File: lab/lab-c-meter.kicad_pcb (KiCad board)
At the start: 2 copper layers, 80 x 34.3 mm, 43 parts, among them J1 IN, J2 Barrel_Jack_Switch, J3 Conn_01x04, J4 USB_B_Mini, J5 PB, J6 PC, J7 PD, SW1 SW_Push, SW2 SW_Push, U1 LM324, U2 L7805, U3 ATmega8-16AU, Y1 16MHz

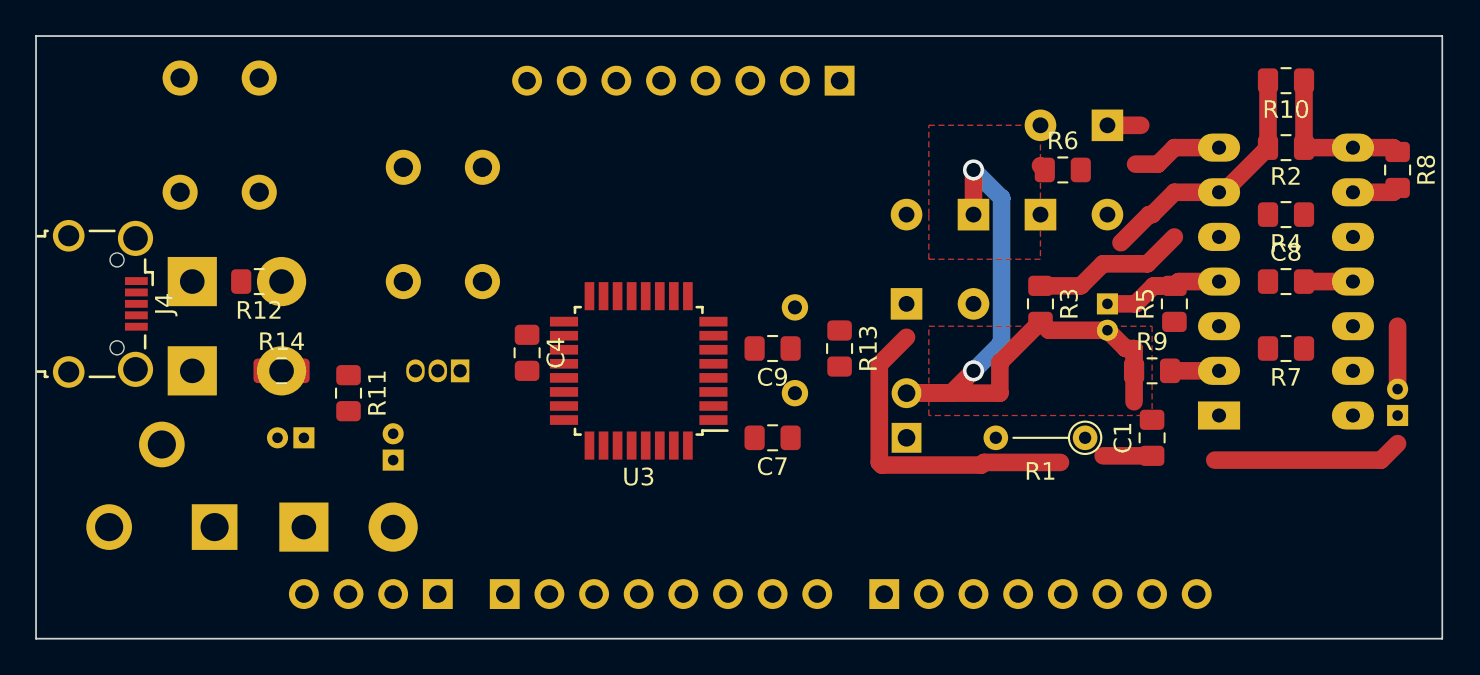
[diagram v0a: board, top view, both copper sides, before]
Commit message: Finished
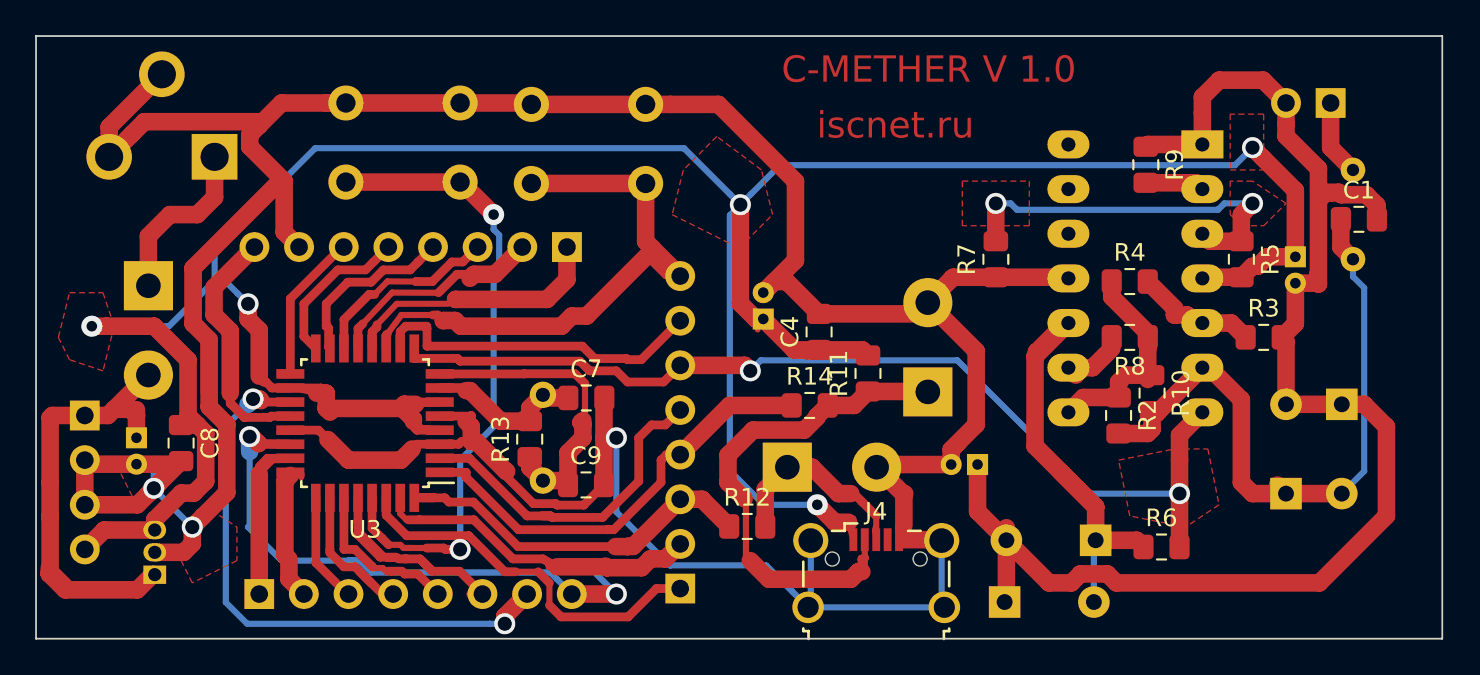
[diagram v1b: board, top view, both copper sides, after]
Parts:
- R1: moved to B.Cu
- moved C8 63.5 mm to (27.3, 52.4), turned to 270 degrees
- moved J4 46.6 mm to (66.9, 59.8), turned to 0 degrees
- moved D7 41.9 mm to (69.8, 49.5), turned to 90 degrees
- moved D6 35.5 mm to (61.8, 53.7)
- moved R12 31.1 mm to (59.5, 57.1), turned to 0 degrees
- moved J1 30.7 mm to (92.7, 33.0), turned to 90 degrees
- moved R14 30.1 mm to (63.1, 50.2)
- moved R11 29.6 mm to (66.4, 48.4), turned to 90 degrees
- moved C5 27.0 mm to (60.4, 45.3), turned to 90 degrees
- moved D1 24.1 mm to (90.2, 55.2)
- moved C3 24.1 mm to (72.6, 53.6), turned to 180 degrees
- moved D3 23.6 mm to (79.3, 57.9), turned to 180 degrees
- moved D2 23.6 mm to (93.3, 50.2)
- moved J3 22.5 mm to (21.8, 50.8), turned to 180 degrees
- moved R6 22.2 mm to (83.1, 58.3)
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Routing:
- net GND: track 6.37 -> 237.9 mm, vias 0 -> 3
- net +5V: track 6.88 -> 182.0 mm, vias 0 -> 5
- net CNT: track 5.14 -> 57.2 mm, vias 0 -> 2
- net PD7: track 0.00 -> 43.8 mm
- net Net-(SW1-Pad2): track 0.00 -> 39.2 mm, vias 0 -> 2
- net MID: track 50.1 -> 87.6 mm, vias 2 -> 0
- net VIN: track 0.00 -> 36.9 mm
- net ADC6: track 0.00 -> 35.8 mm, vias 0 -> 2
- net ADC7: track 0.00 -> 35.3 mm, vias 0 -> 2
- net Net-(D3-Pad1): track 2.25 -> 31.5 mm
- net Net-(D7-Pad1): track 0.00 -> 29.2 mm
- net D-: track 0.00 -> 26.5 mm
- net D+: track 0.00 -> 23.6 mm
- net PD0: track 0.00 -> 22.7 mm
- net PD1: track 0.00 -> 22.3 mm
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- added copper zone on F.Cu, net +5V
- added copper zone on F.Cu, net CNT
- added copper zone on F.Cu, net GND
- added copper zone on F.Cu, net Net-(R5-Pad1)
- removed copper zone on F.Cu, net MID
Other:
- board text added: "C-METHER V 1.0"
- board text added: "iscnet.ru"

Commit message: Production
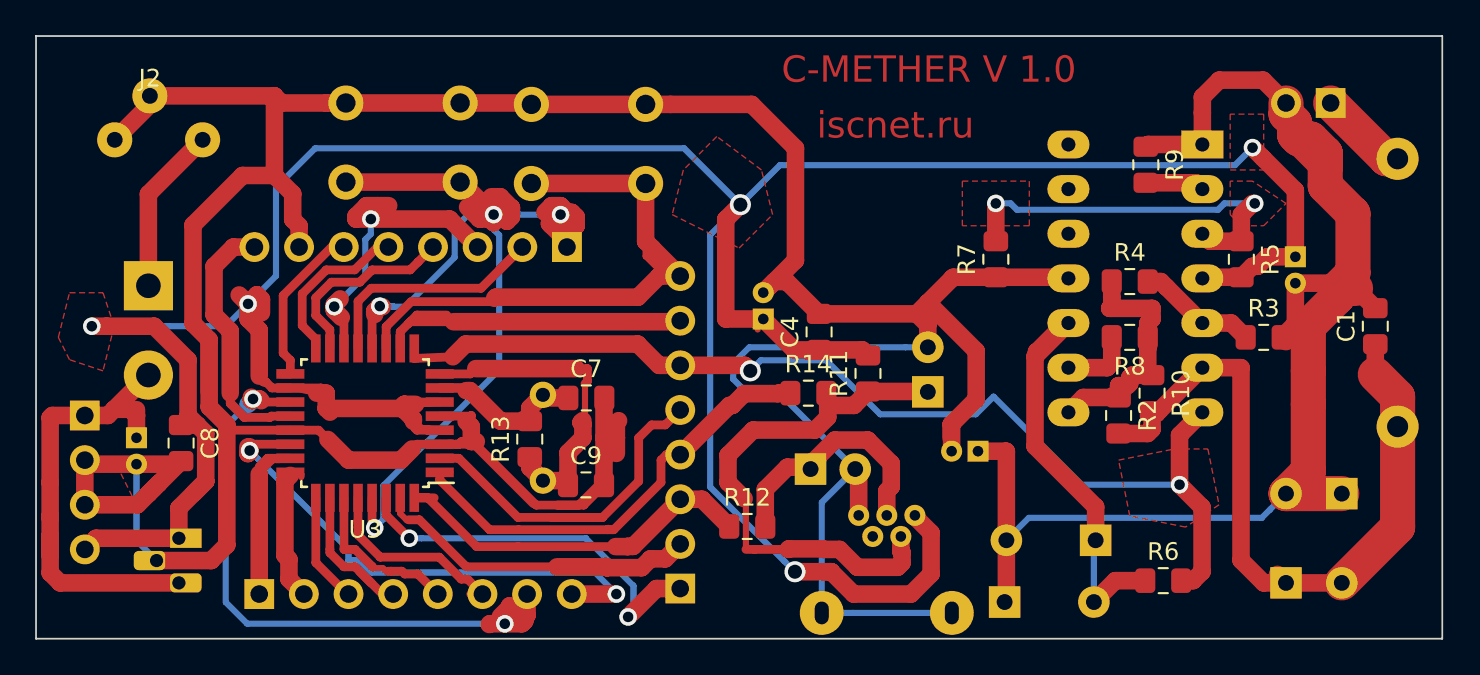
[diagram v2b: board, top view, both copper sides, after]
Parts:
- D6: footprint Diode_THT:D_5W_P5.08mm_Vertical_KathodeUp -> Diode_THT:D_A-405_P2.54mm_Vertical_AnodeUp
- D7: footprint Diode_THT:D_5W_P5.08mm_Vertical_KathodeUp -> Diode_THT:D_A-405_P2.54mm_Vertical_KathodeUp
- J2: footprint Connector_BarrelJack:BarrelJack_CUI_PJ-102AH_Horizontal -> local:Barrel-little-11mm-x-5mm; moved to F.Cu
- J4: footprint Connector_USB:USB_Micro-B_Wuerth_629105150521_CircularHoles -> local:USB-mini-S2126.12010-Circular; moved to B.Cu
- R1: footprint Resistor_THT:R_Axial_DIN0204_L3.6mm_D1.6mm_P5.08mm_Vertical -> Resistor_THT:R_Axial_DIN0414_L11.9mm_D4.5mm_P15.24mm_Horizontal
- U2: value L7805 -> L78L05_TO92; footprint Package_TO_SOT_THT:TO-92S -> Package_TO_SOT_THT:TO-92_HandSolder
- moved R1 9.86 mm to (96.5, 51.4)
- moved J2 6.19 mm to (25.5, 31.1), turned to 0 degrees
- moved C1 6.15 mm to (95.2, 45.7), turned to 90 degrees
- moved J4 5.29 mm to (67.1, 54.5), turned to 180 degrees
- moved D1 5.08 mm to (90.2, 60.3)
- moved D2 5.08 mm to (93.3, 55.2)
- moved U2 2.49 mm to (27.2, 57.8), turned to 270 degrees
- moved R6 1.92 mm to (83.2, 60.2)
- moved D6 1.33 mm to (63.1, 53.8)
- moved C3 0.76 mm to (72.6, 52.8)
- moved R14 0.70 mm to (63.0, 49.5)
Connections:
- U2 pad 1: VIN -> +5V
- U2 pad 3: +5V -> VIN
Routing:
- net +5V: track 182.0 -> 203.2 mm
- net Net-(J5-Pad1): track 15.7 -> 26.4 mm, vias 0 -> 2
- net Net-(J5-Pad3): track 11.0 -> 19.6 mm, vias 0 -> 2
- net PD7: track 43.8 -> 38.6 mm
- net VIN: track 36.9 -> 31.8 mm
- net MID: track 87.6 -> 82.6 mm
- net Net-(C1-Pad1): track 37.6 -> 42.5 mm
- net ADC7: track 35.3 -> 31.1 mm
- net ADC6: track 35.8 -> 40.0 mm
- net PC5: track 15.7 -> 11.6 mm
- net CNT: track 57.2 -> 61.0 mm
- net PD1: track 22.3 -> 18.8 mm
- net Net-(R10-Pad1): track 12.7 -> 15.2 mm
- net Net-(D3-Pad1): track 31.5 -> 29.2 mm
- net PD4: track 19.7 -> 21.9 mm
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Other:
- net class Default: via_dia 1.2 -> 1; via_drill 0.8 -> 0.6
- net class mid: via_dia 1.2 -> 1; via_drill 0.8 -> 0.6
- net class wide: via_dia 1.2 -> 1; via_drill 0.8 -> 0.6
